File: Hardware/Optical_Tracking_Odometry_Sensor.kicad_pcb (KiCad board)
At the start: 2 copper layers, 25.4 x 25.4 mm, 55 parts, among them J3 CONN_06NO_SILK_NO_POP, Q1 100mA/20V/3.8Ω, Q2 100mA/20V/3.8Ω, U1 PAA5160E1-Q, U2 LSM6DS0, U3 STM32C011F6U6, U4 RT9080-18GJ5

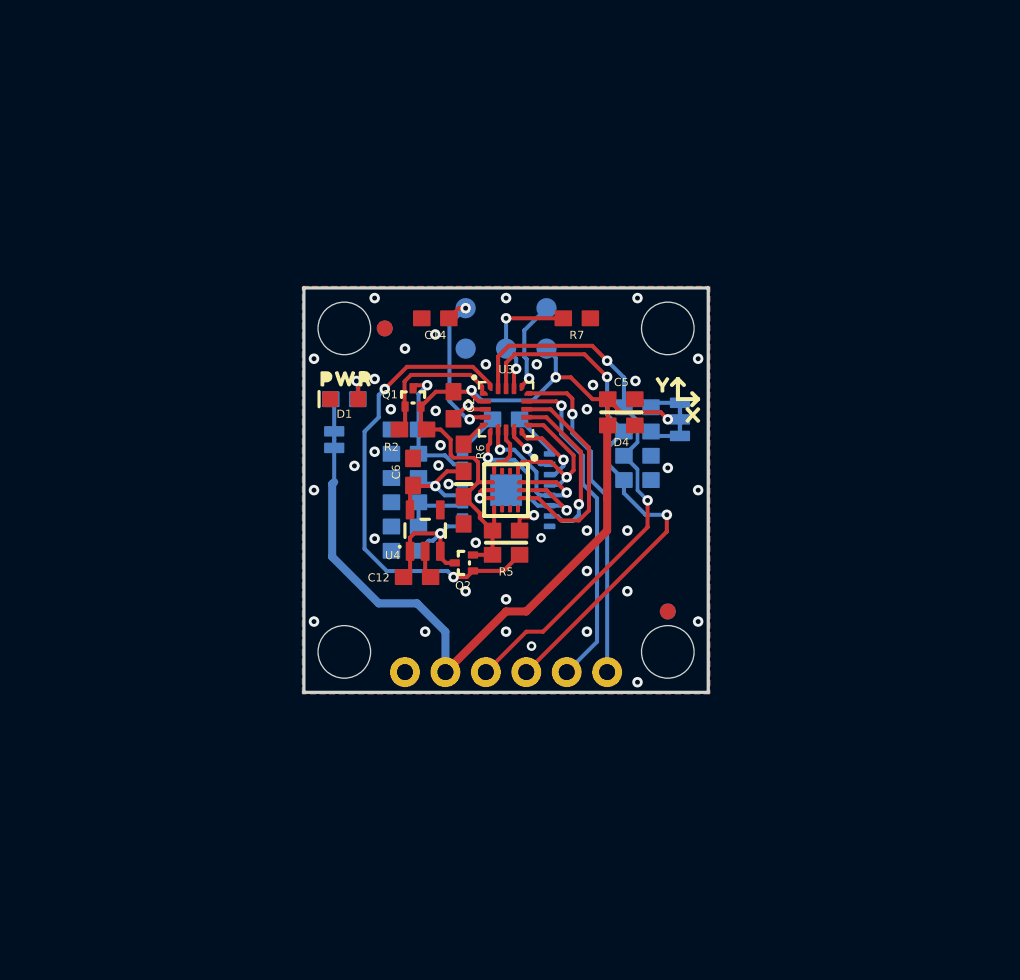
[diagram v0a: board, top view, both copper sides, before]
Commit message: Improvements
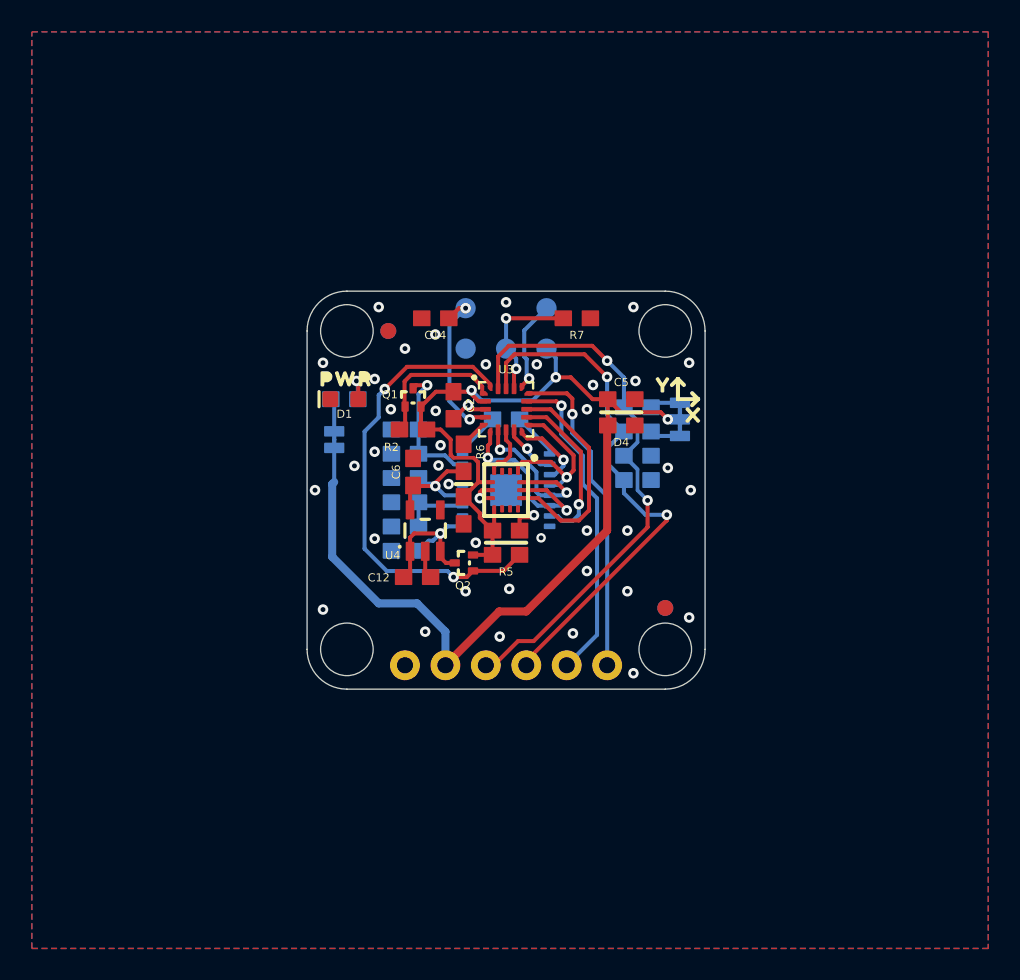
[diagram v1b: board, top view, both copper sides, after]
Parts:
- moved J3 0.43 mm to (142.2, 116.0)
- moved FD1 0.27 mm to (141.1, 95.0)
- moved FD2 0.27 mm to (141.1, 95.0)
- moved FD3 0.27 mm to (158.5, 112.4)
- moved FD4 0.27 mm to (158.5, 112.4)
- moved H2 0.23 mm to (138.5, 95.0)
- moved H3 0.23 mm to (158.5, 95.0)
- moved H1 0.23 mm to (138.5, 115.0)
- moved H4 0.23 mm to (158.5, 115.0)
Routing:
- net 3.3V: track 79.3 -> 78.7 mm
- net GND: vias 42 -> 41
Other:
- board size 25.4 x 25.4 mm -> 25 x 25 mm
